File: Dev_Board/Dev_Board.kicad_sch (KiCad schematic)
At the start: 24 parts, among them J1 Conn_01x04, J2 Conn_01x04

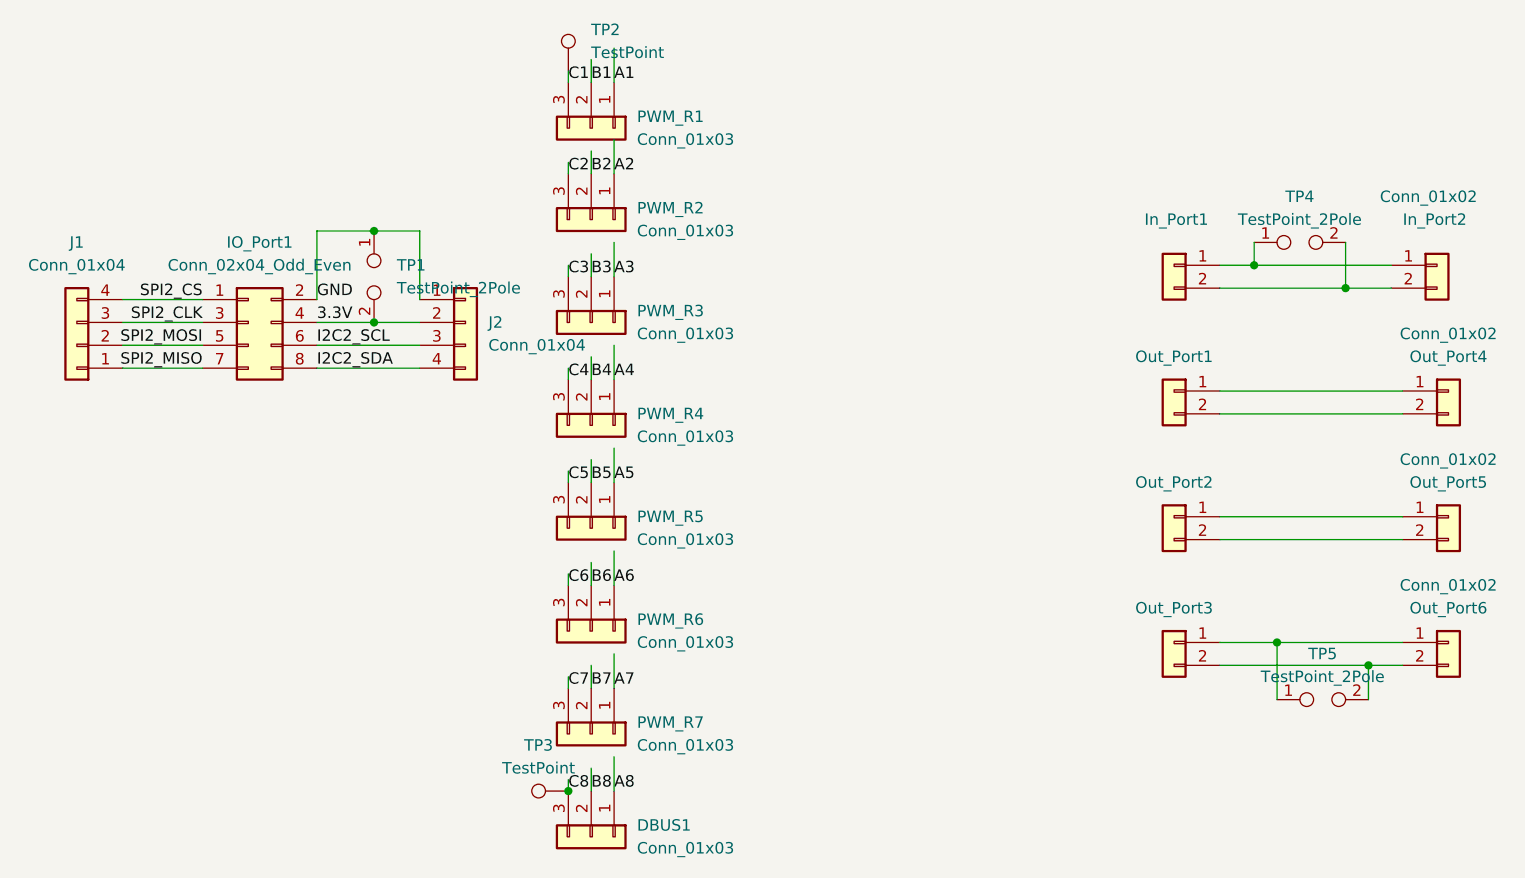
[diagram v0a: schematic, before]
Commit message: 02/09/2024 sch
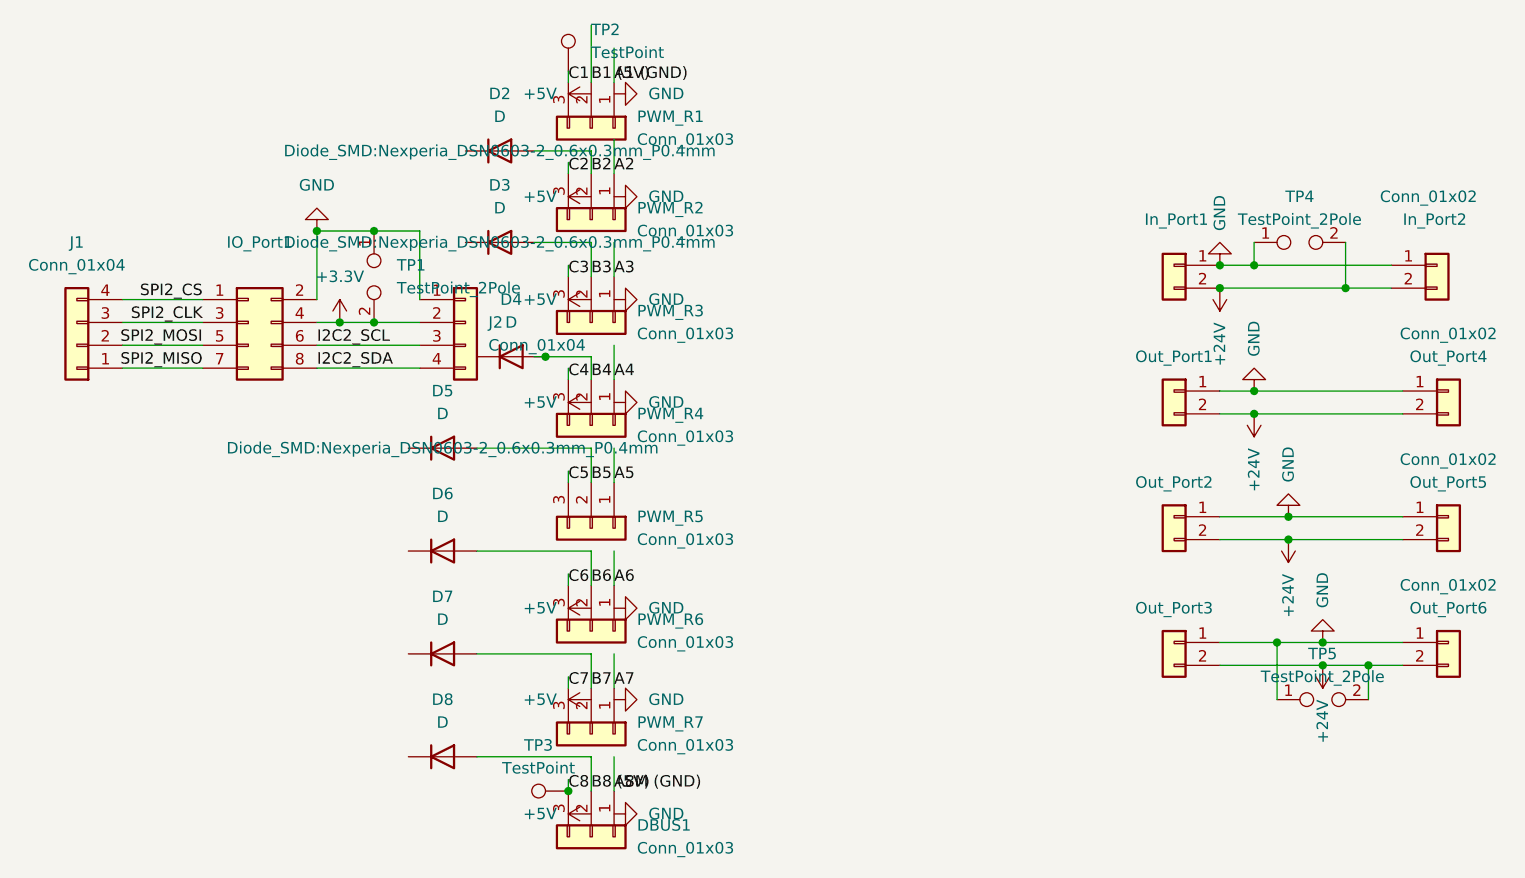
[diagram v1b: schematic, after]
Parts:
- added D2, D3, D4, D5, D6, D7, D8: D, Diode_SMD:Nexperia_DSN0603-2_0.6x0.3mm_P0.4mm, symbol Device:D
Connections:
- net B2: now also D2.2 (A)
- net B3: now also D3.2 (A)
- net B4: now also D4.2 (A)
- net B5: now also D5.2 (A)
- net B6: now also D6.2 (A)
- net B7: now also D7.2 (A)
- net GND: now also In_Port1.1 (Pin_1), In_Port2.1 (Pin_1), Out_Port1.1 (Pin_1), Out_Port2.1 (Pin_1), Out_Port3.1 (Pin_1), Out_Port4.1 (Pin_1), Out_Port5.1 (Pin_1), Out_Port6.1 (Pin_1), TP4.1, TP5.1
- net +24V: now reaches Out_Port1.2 (Pin_2), Out_Port4.2 (Pin_2)
- net +24V: now also In_Port1.2 (Pin_2), In_Port2.2 (Pin_2), Out_Port2.2 (Pin_2), Out_Port3.2 (Pin_2), Out_Port5.2 (Pin_2), Out_Port6.2 (Pin_2), TP4.2, TP5.2
- net 3.3V renamed +3.3V
- net A1 renamed A1 (GND)
- net A8 renamed A8M (GND)
- net B1 renamed B1 (5V)
- net B8 renamed B8 (5V)
- net B8 (5V): now also D8.2 (A)
